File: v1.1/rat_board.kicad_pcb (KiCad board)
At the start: 2 copper layers, 78.7 x 109.2 mm, 23 parts, among them J1 Conn_01x02, J2 Conn_01x04, J3 Conn_01x02, J4 Conn_01x02, J5 Conn_01x02, J6 Conn_01x03, J7 Conn_01x02, J8 Conn_01x02, SW1 SW_SPDT, SW2 SW_Push, U2 DRV8835

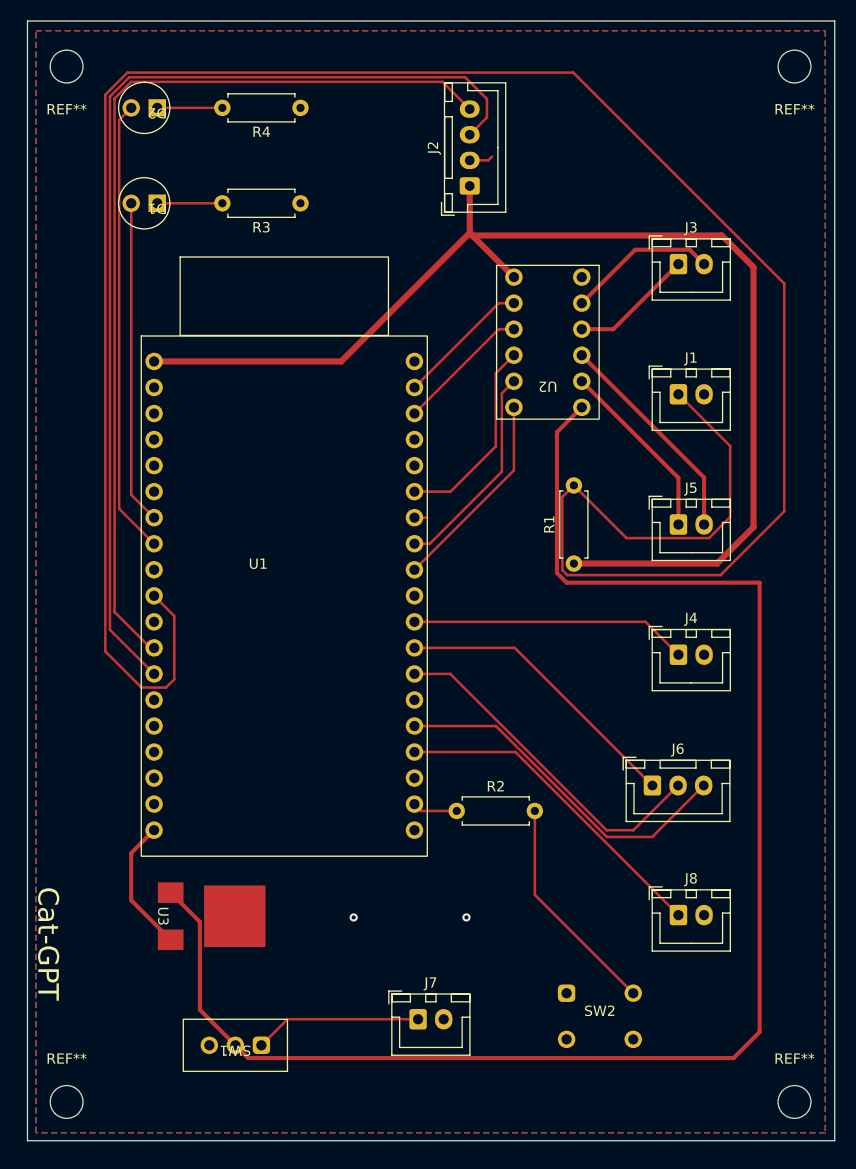
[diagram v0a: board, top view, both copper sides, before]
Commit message: feat: 基板できた！
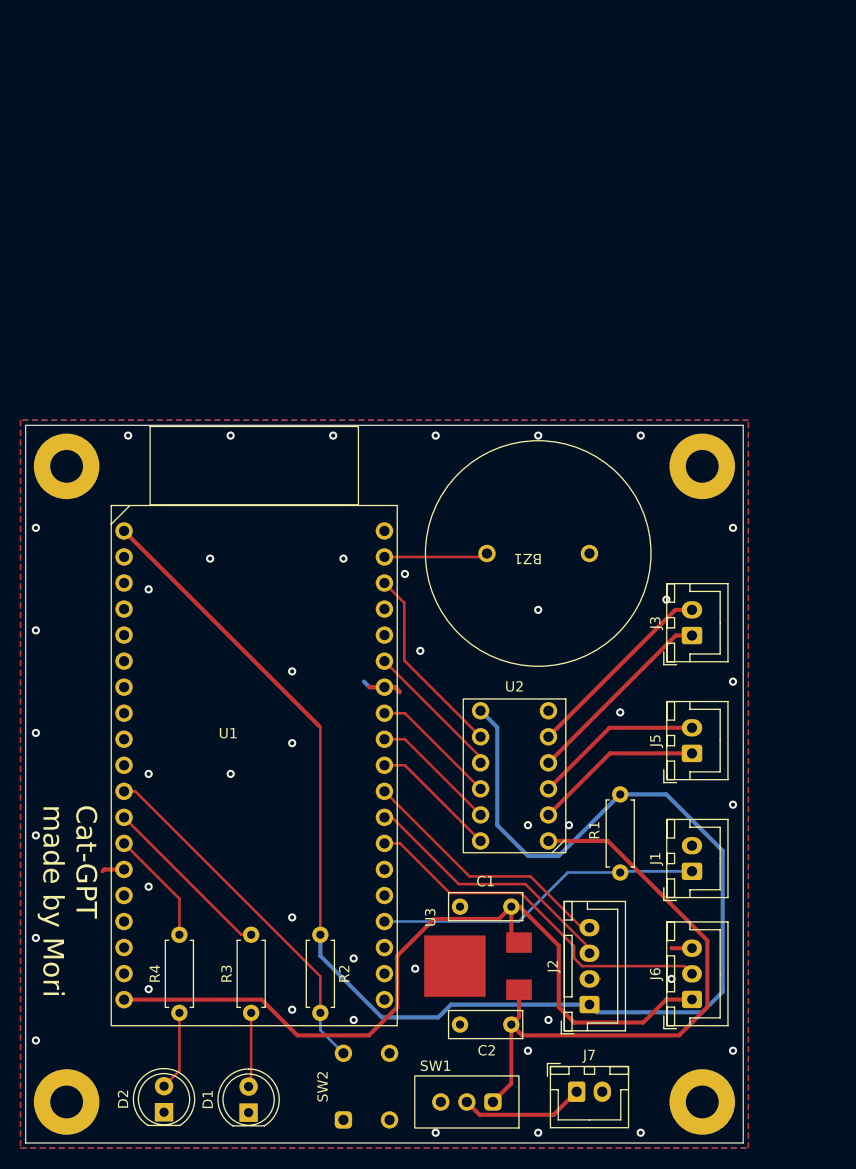
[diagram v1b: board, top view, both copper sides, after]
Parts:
- removed J4, J8: Conn_01x02, Connector_JST:JST_XH_B2B-XH-A_1x02_P2.50mm_Vertical
- removed REF** (x4): MountingHole_3.2mm_M3, MountingHole:MountingHole_3.2mm_M3
- added BZ1: Buzzer, mori:PKM22EPP-40, F.Cu at (154.0, 87.5)
- added C1: 2.2u, Capacitor_THT:C_Disc_D7.0mm_W2.5mm_P5.00mm, F.Cu at (151.4, 122.0)
- added C2: 0.33u, Capacitor_THT:C_Disc_D7.0mm_W2.5mm_P5.00mm, F.Cu at (146.4, 133.4)
- added H1: MountingHole_Pad, MountingHole:MountingHole_3.2mm_M3_Pad, F.Cu at (108.0, 79.0)
- added H2: MountingHole_Pad, MountingHole:MountingHole_3.2mm_M3_Pad, F.Cu at (170.0, 79.0)
- added H3: MountingHole_Pad, MountingHole:MountingHole_3.2mm_M3_Pad, F.Cu at (170.0, 141.0)
- added H4: MountingHole_Pad, MountingHole:MountingHole_3.2mm_M3_Pad, F.Cu at (108.0, 141.0)
- D1: value LED -> LED BLUE; footprint mori:LED -> LED_THT:LED_D5.0mm
- D2: value LED -> LED WHITE; footprint mori:LED -> LED_THT:LED_D5.0mm
- R3, R4: value 110 -> 470
- U3: value ~ -> NJM2845DL-05
- moved D2 98.0 mm to (117.5, 142.0), turned to 90 degrees
- moved D1 89.1 mm to (125.8, 142.0), turned to 90 degrees
- moved R4 89.1 mm to (119.0, 132.3), turned to 90 degrees
- moved J2 80.7 mm to (159.0, 131.5)
- moved R3 79.1 mm to (126.0, 132.3), turned to 90 degrees
- moved J1 46.5 mm to (169.0, 118.5), turned to 90 degrees
- moved U2 42.4 mm to (151.7, 113.0)
- moved U3 36.8 mm to (153.4, 127.8), turned to 90 degrees
- moved J3 36.3 mm to (169.0, 95.5), turned to 90 degrees
- moved SW2 23.8 mm to (137.2, 139.5), turned to 90 degrees
- moved SW1 23.2 mm to (147.0, 141.0)
- moved R1 23.0 mm to (162.0, 111.0), turned to -90 degrees
- moved J5 22.4 mm to (169.0, 107.0), turned to 90 degrees
- moved J6 21.2 mm to (169.0, 131.0), turned to 90 degrees
- moved R2 18.0 mm to (132.8, 124.7), turned to -90 degrees
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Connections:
- net Net-(J6-Pin_2) renamed RGBLED
- D1 pad 1: Net-(D1-K) -> GND
- D2 pad 1: Net-(D2-K) -> GND
- J1 pad 1: Net-(J1-Pin_1) -> LIMIT_SW
- J2 pad 1: 3.3V -> +3.3V
- J6 pad 1: Net-(J6-Pin_1) -> +5V
- J6 pad 3: Net-(J6-Pin_3) -> GND
- J7 pad 1: +6V -> Net-(J7-Pin_1)
- R1 pad 1: 3.3V -> +3.3V
- R1 pad 2: Net-(J1-Pin_1) -> LIMIT_SW
- R2 pad 1: Net-(U1-IO7) -> +3.3V
- R2 pad 2: Net-(R2-Pad2) -> SW
- R3 pad 1: GND -> Net-(D1-A)
- R3 pad 2: Net-(D1-K) -> LED_A
- R4 pad 1: GND -> Net-(D2-A)
- R4 pad 2: Net-(D2-K) -> LED_B
- SW1 pad 1: +6V -> VCC
- SW1 pad 2: Net-(SW1-B) -> Net-(J7-Pin_1)
- SW2 pad 2: Net-(R2-Pad2) -> SW
- U1 pad 1: 3.3V -> +3.3V
- U1 pad 10: Net-(J1-Pin_1) -> unconnected-(U1-IO26-Pad10)
- U1 pad 11: unconnected-(U1-IO27-Pad11) -> SW
- U1 pad 12: SCL -> LED_A
- U1 pad 13: SDA -> LED_B
- U1 pad 19: Net-(U1-5V) -> +5V
- U1 pad 21: Net-(U1-IO7) -> unconnected-(U1-IO7-Pad21)
- U1 pad 23: Net-(J8-Pin_1) -> LIMIT_SW
- U1 pad 24: Net-(J6-Pin_3) -> unconnected-(U1-IO2-Pad24)
- U1 pad 27: Net-(J6-Pin_1) -> SDA
- U1 pad 28: Net-(J4-Pin_1) -> SCL
- U1 pad 29: unconnected-(U1-IO5-Pad29) -> BIN2
- U1 pad 30: BIN2 -> BIN1
- U1 pad 31: BIN1 -> AIN2
- U1 pad 33: AIN2 -> AIN1
- U1 pad 36: AIN1 -> MODE
- U1 pad 37: MODE -> BUZZER
- U1 pad 7: Net-(D1-A) -> unconnected-(U1-IO32-Pad7)
- U1 pad 8: Net-(D2-A) -> unconnected-(U1-IO33-Pad8)
- U2 pad 1: Net-(SW1-B) -> VCC
- U2 pad 7: 3.3V -> +3.3V
- U3 pad 1: Net-(SW1-B) -> VCC
- U3 pad 3: Net-(U1-5V) -> +5V
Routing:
- net Net-(J1-Pin_1): track 235.1 -> 0.00 mm
- net Net-(SW1-B): track 151.4 -> 0.00 mm
- net +3.3V: track 0.00 -> 146.4 mm
- net 3.3V: track 119.7 -> 0.00 mm
- net +5V: track 0.00 -> 77.9 mm
- net SDA: track 100.7 -> 25.8 mm
- net SCL: track 92.4 -> 25.5 mm
- net VCC: track 0.00 -> 58.7 mm
- net Net-(D2-A): track 44.4 -> 7.77 mm
- net SW: track 0.00 -> 35.1 mm
- net Net-(J6-Pin_3): track 34.8 -> 0.00 mm
- net Net-(J8-Pin_1): track 32.3 -> 0.00 mm
- net LIMIT_SW: track 0.00 -> 32.2 mm
- net Net-(J6-Pin_1): track 28.8 -> 0.00 mm
- net Net-(J4-Pin_1): track 27.1 -> 0.00 mm
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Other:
- board size 78.7 x 109.2 mm -> 70 x 70 mm
- board text added: "Cat-GPT made by Mori"
- board text removed: "Cat-GPT"
- board text removed: "Tool Play Ground"
